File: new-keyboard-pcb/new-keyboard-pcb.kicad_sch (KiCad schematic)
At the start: 23 parts, among them J1 Conn_ARM_JTAG_SWD_10, SW100 SW_Push_Dual, U1 PRTR5V0U2X, U2 STM32F072CBTx, U3 AP2112K-3.3, Y1 8MHz

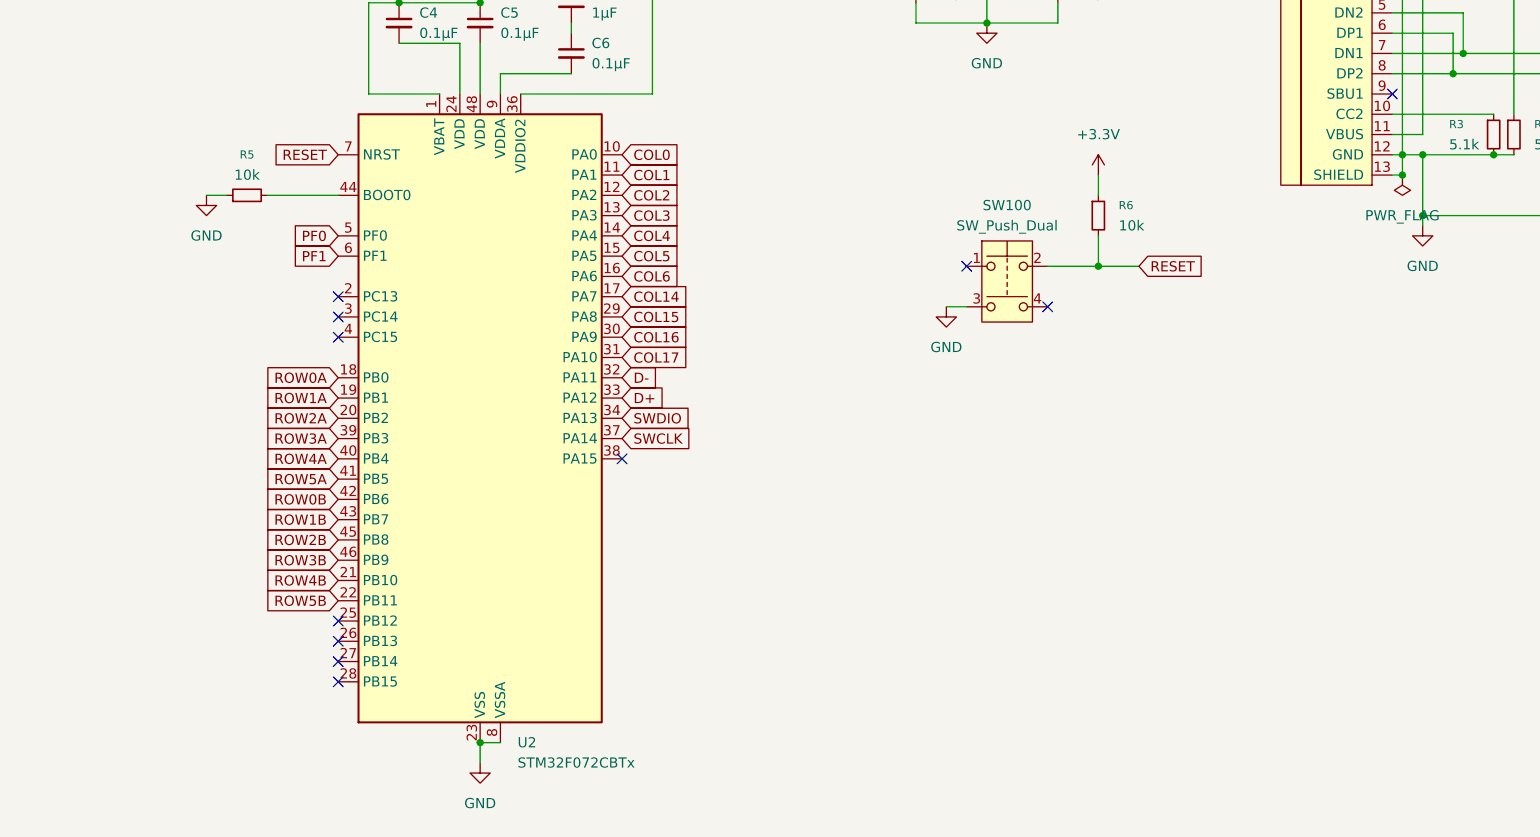
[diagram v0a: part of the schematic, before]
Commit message: midway correcting hotswap sockets
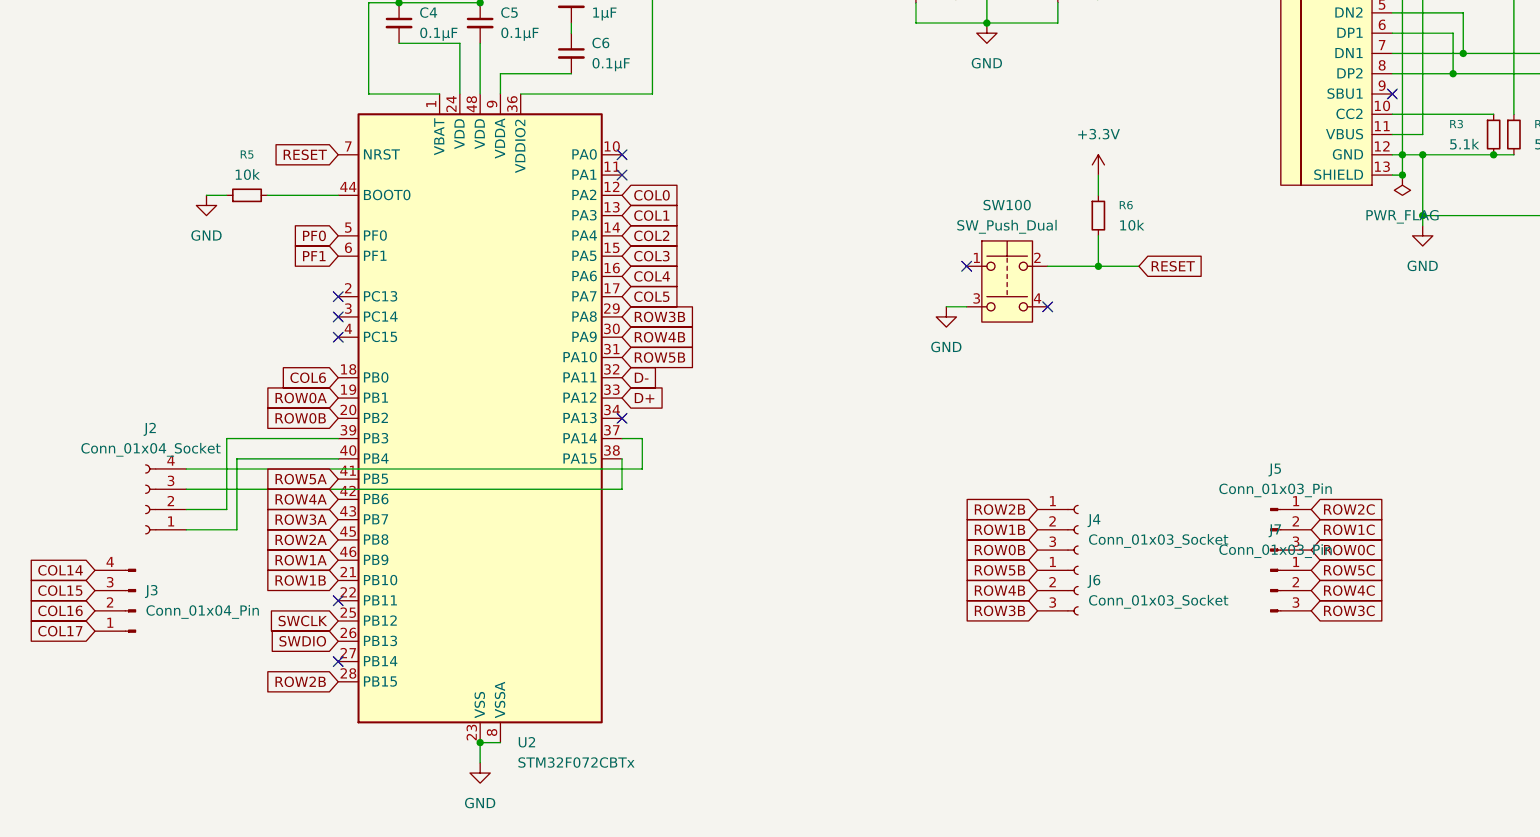
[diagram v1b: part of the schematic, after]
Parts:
- added J2: Conn_01x04_Socket, pogo_conn_4_pins:686L0421350120E, symbol Connector:Conn_01x04_Socket
- added J3: Conn_01x04_Pin, pogo_conn_4_pins:685L0421250110E, symbol Connector:Conn_01x04_Pin
- added J4, J6: Conn_01x03_Socket, pogo_conn_3_pins:685F0321351124E, symbol Connector:Conn_01x03_Socket
- added J5, J7: Conn_01x03_Pin, pogo_conn_3_pins:685F0321350124E, symbol Connector:Conn_01x03_Pin
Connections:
- net COL0: now also U2.12 (PA2); no longer U2.10 (PA0)
- net COL1: now also U2.13 (PA3); no longer U2.11 (PA1)
- net COL14: now also J3.4 (Pin_4); no longer U2.17 (PA7)
- net COL15: now also J3.3 (Pin_3); no longer U2.29 (PA8)
- net COL16: now also J3.2 (Pin_2); no longer U2.30 (PA9)
- net COL17: now also J3.1 (Pin_1); no longer U2.31 (PA10)
- net COL2: now also U2.14 (PA4); no longer U2.12 (PA2)
- net COL3: now also U2.15 (PA5); no longer U2.13 (PA3)
- net COL4: now also U2.16 (PA6); no longer U2.14 (PA4)
- net COL5: now also U2.17 (PA7); no longer U2.15 (PA5)
- net COL6: now also U2.18 (PB0); no longer U2.16 (PA6)
- net ROW0A: now also U2.19 (PB1); no longer U2.18 (PB0)
- net ROW0B: now also U2.20 (PB2), J4.3 (Pin_3); no longer U2.42 (PB6)
- net ROW1A: now also U2.46 (PB9); no longer U2.19 (PB1)
- net ROW1B: now also U2.21 (PB10), J4.2 (Pin_2); no longer U2.43 (PB7)
- net ROW2A: now also U2.45 (PB8); no longer U2.20 (PB2)
- net ROW2B: now also U2.28 (PB15), J4.1 (Pin_1); no longer U2.45 (PB8)
- net ROW3A: now also U2.43 (PB7); no longer U2.39 (PB3)
- net ROW3B: now also U2.29 (PA8), J6.3 (Pin_3); no longer U2.46 (PB9)
- net ROW4A: now also U2.42 (PB6); no longer U2.40 (PB4)
- net ROW4B: now also U2.30 (PA9), J6.2 (Pin_2); no longer U2.21 (PB10)
- net ROW5B: now also U2.31 (PA10), J6.1 (Pin_1); no longer U2.22 (PB11)
- net SWCLK: now also U2.25 (PB12); no longer U2.37 (PA14)
- net SWDIO: now also U2.26 (PB13); no longer U2.34 (PA13)
- net at U2.38 (PA15): now also J2.3 (Pin_3)
- new net: J2.4 (Pin_4), U2.37 (PA14)
- new net: J2.2 (Pin_2), U2.39 (PB3)
- new net: J2.1 (Pin_1), U2.40 (PB4)
- new net ROW0C: J5.3 (Pin_3)
- new net ROW1C: J5.2 (Pin_2)
- new net ROW2C: J5.1 (Pin_1)
- new net ROW3C: J7.3 (Pin_3)
- new net ROW4C: J7.2 (Pin_2)
- new net ROW5C: J7.1 (Pin_1)
